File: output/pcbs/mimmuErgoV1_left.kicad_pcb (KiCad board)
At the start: 2 copper layers, 144.7 x 96.9 mm, 47 parts

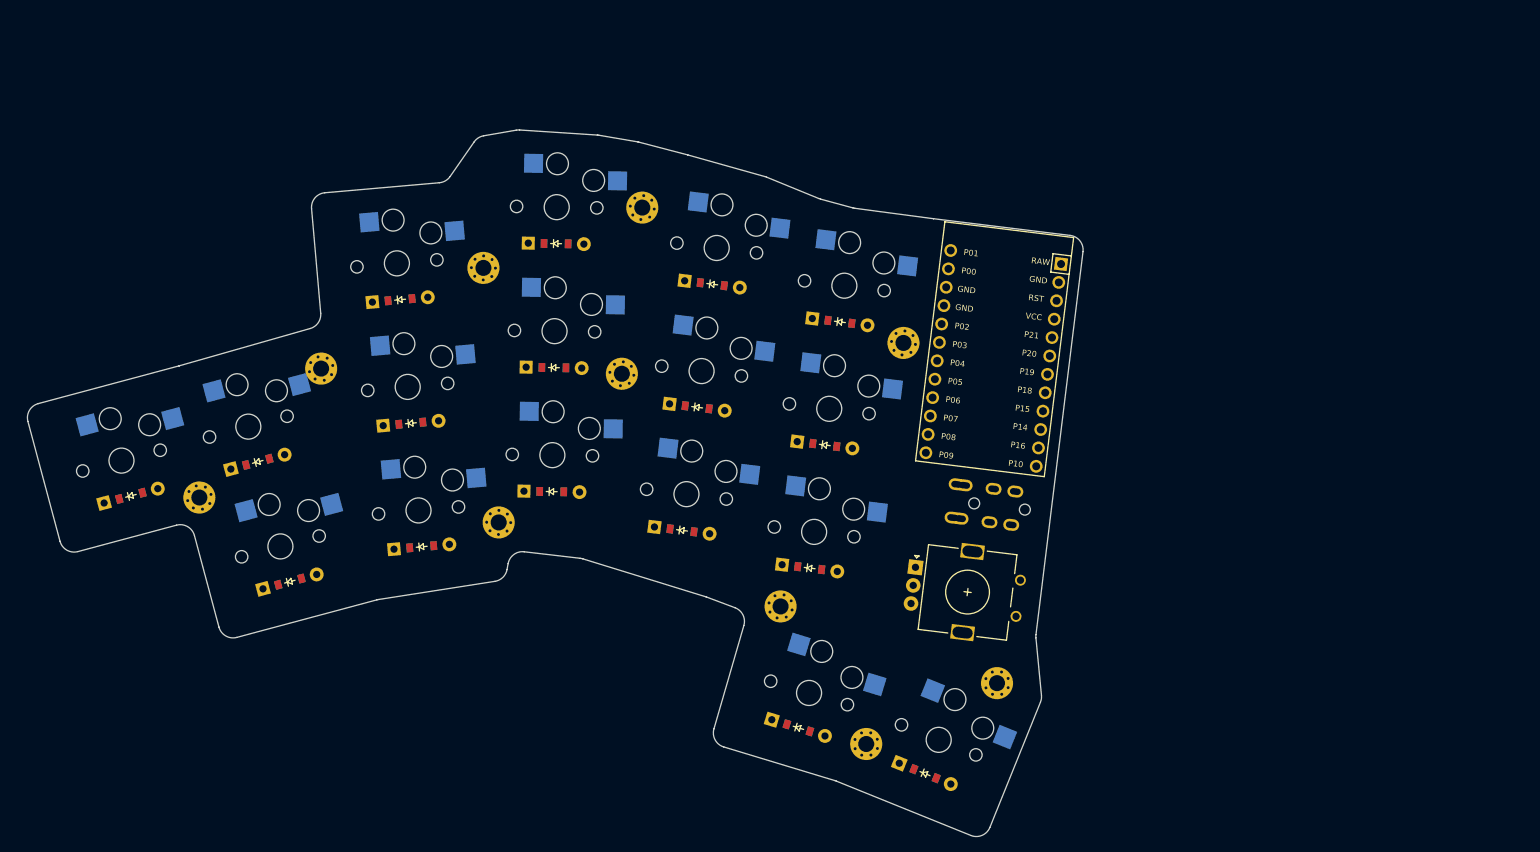
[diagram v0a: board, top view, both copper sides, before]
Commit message: Add files via upload
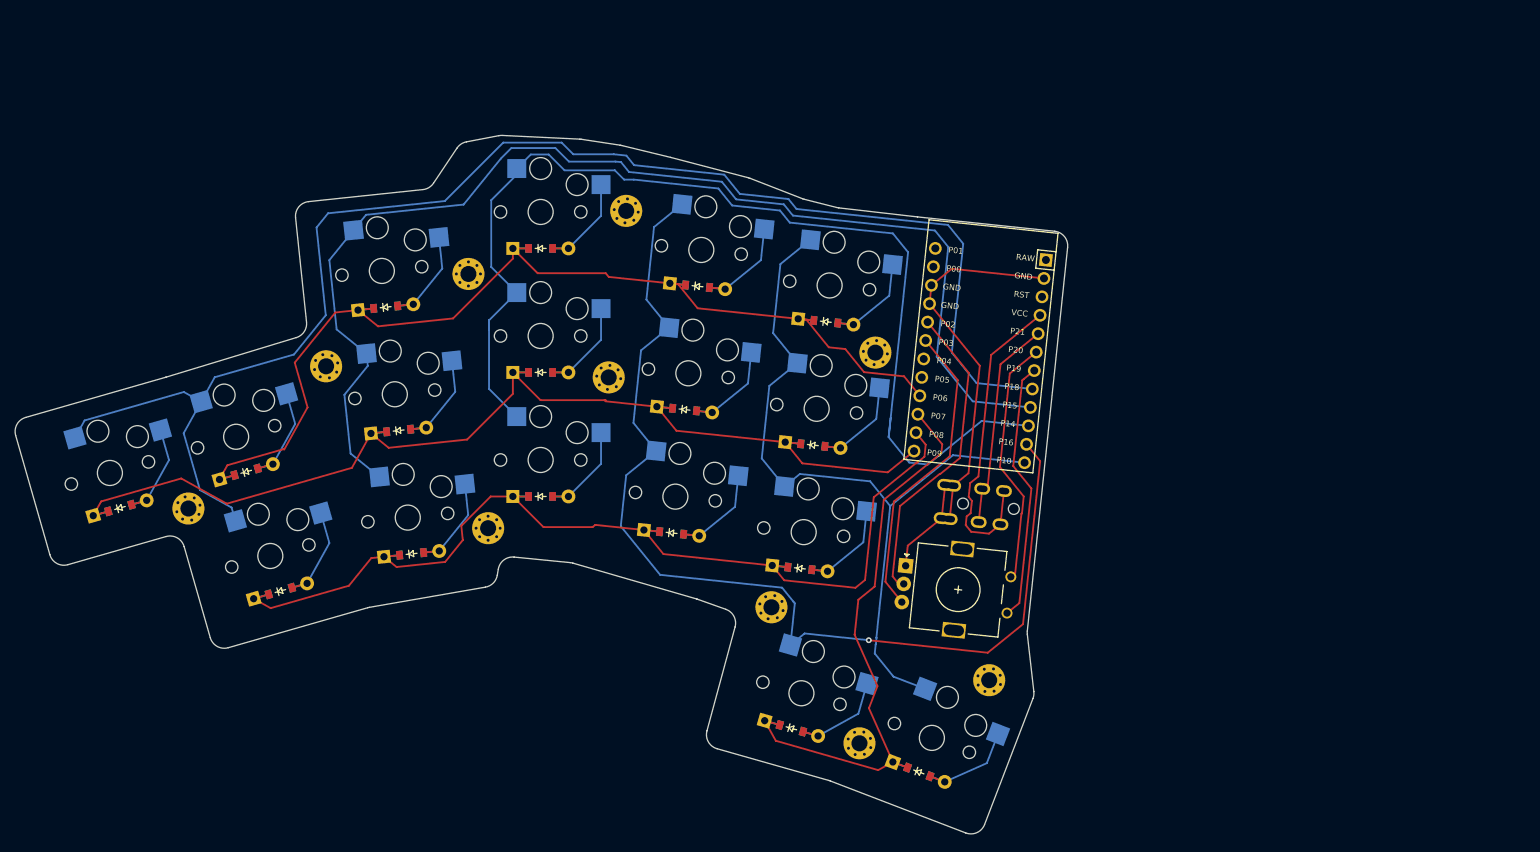
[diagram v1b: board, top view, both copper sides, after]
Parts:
- moved _3 4.07 mm to (181.6, 153.7), turned to -6 degrees
- moved S3 2.32 mm to (76.7, 170.2), turned to 16 degrees
- moved S6 2.31 mm to (114.0, 142.5), turned to 6 degrees
- moved S9 2.30 mm to (135.7, 134.4), turned to 0 degrees
- moved _2 2.25 mm to (147.5, 134.3), turned to -6 degrees
- moved D3 2.25 mm to (78.1, 175.0), turned to 16 degrees
- moved D6 2.23 mm to (114.5, 147.5), turned to 6 degrees
- moved _1 2.22 mm to (125.8, 142.9), turned to 0 degrees
- moved D9 2.21 mm to (135.7, 139.4), turned to 0 degrees
- moved S2 2.17 mm to (94.0, 165.2), turned to 16 degrees
- moved S12 2.13 mm to (157.8, 139.6), turned to -6 degrees
- moved _9 2.13 mm to (87.4, 175.0), turned to 16 degrees
- moved D2 2.09 mm to (95.4, 170.0), turned to 16 degrees
- moved D12 2.04 mm to (157.2, 144.6), turned to -6 degrees
- moved S5 2.04 mm to (115.7, 159.4), turned to 6 degrees
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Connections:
- D2 pad 1: P9 -> P6
- D3 pad 1: P6 -> P9
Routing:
- net P18: track 0.00 -> 199.4 mm
- net P15: track 0.00 -> 161.8 mm
- net P9: track 0.00 -> 152.3 mm
- net P14: track 0.00 -> 151.8 mm
- net P6: track 0.00 -> 147.5 mm
- net P16: track 0.00 -> 145.4 mm, vias 0 -> 1
- net P8: track 0.00 -> 142.8 mm
- net P10: track 0.00 -> 106.8 mm
- net P7: track 0.00 -> 84.0 mm
- net GND: track 0.00 -> 67.5 mm
- net P2: track 0.00 -> 43.7 mm
- net VCC: track 0.00 -> 43.3 mm
- net P3: track 0.00 -> 42.0 mm
- net P19: track 0.00 -> 35.9 mm
- net P20: track 0.00 -> 34.1 mm
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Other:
- board size 144.7 x 96.9 mm -> 144.3 x 95.7 mm
- net class Default removed

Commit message: finalize
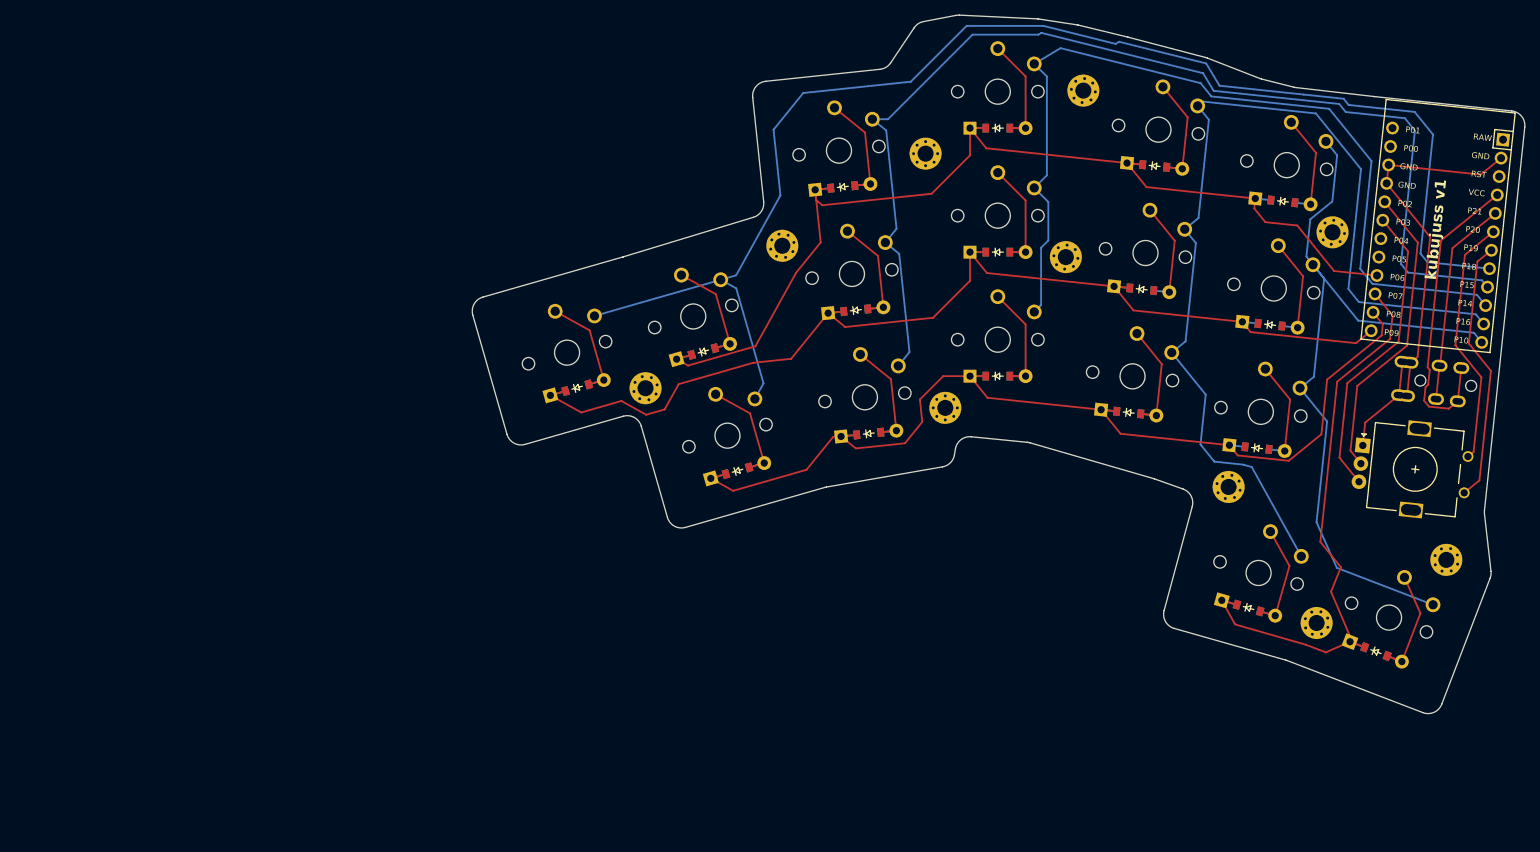
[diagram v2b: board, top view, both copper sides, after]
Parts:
- moved TRRS1 64.9 mm to (264.6, 160.7)
- moved D2 64.8 mm to (158.0, 153.5)
- moved S1 64.8 mm to (161.3, 165.1)
- moved S17 64.8 mm to (252.0, 190.0)
- moved S7 64.8 mm to (198.4, 151.9)
- moved _6 64.8 mm to (230.0, 172.1)
- moved S5 64.8 mm to (178.4, 142.9)
- moved _9 64.8 mm to (150.1, 158.6)
- moved D10 64.8 mm to (216.3, 161.9)
- moved S8 64.8 mm to (198.4, 134.9)
- moved D8 64.8 mm to (198.4, 139.9)
- moved D12 64.8 mm to (219.9, 128.1)
- moved S2 64.8 mm to (156.7, 148.7)
- moved _1 64.8 mm to (188.5, 126.4)
- moved S13 64.8 mm to (234.5, 161.8)
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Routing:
- net P14: track 151.8 -> 122.6 mm
- net P18: track 199.4 -> 187.2 mm
- net P15: track 161.8 -> 150.9 mm
- net P16: track 145.4 -> 136.3 mm, vias 1 -> 0
- net P8: track 142.8 -> 138.8 mm
- net GND: track 67.5 -> 64.4 mm
- net P2: track 43.7 -> 41.4 mm
- net P9: track 152.3 -> 150.1 mm
- net middle_top: track 14.9 -> 16.8 mm
- net layer_cluster: track 14.9 -> 16.8 mm
- net middle_bottom: track 14.9 -> 16.8 mm
- net pinkie_top: track 14.9 -> 16.8 mm
- net pinkie_bottom: track 14.9 -> 16.8 mm
- net ring_bottom: track 14.9 -> 16.8 mm
- net space_cluster: track 14.9 -> 16.8 mm
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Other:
- outline, holes or cut-outs redrawn
- board text added: "kubujuss v1"
